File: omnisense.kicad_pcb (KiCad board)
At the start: 2 copper layers, 40 x 55 mm, 21 parts, among them J2 USB_C_Receptacle_USB2.0_16P, U1 ESP32-S3-WROOM-1, U3 TLV76133DCY

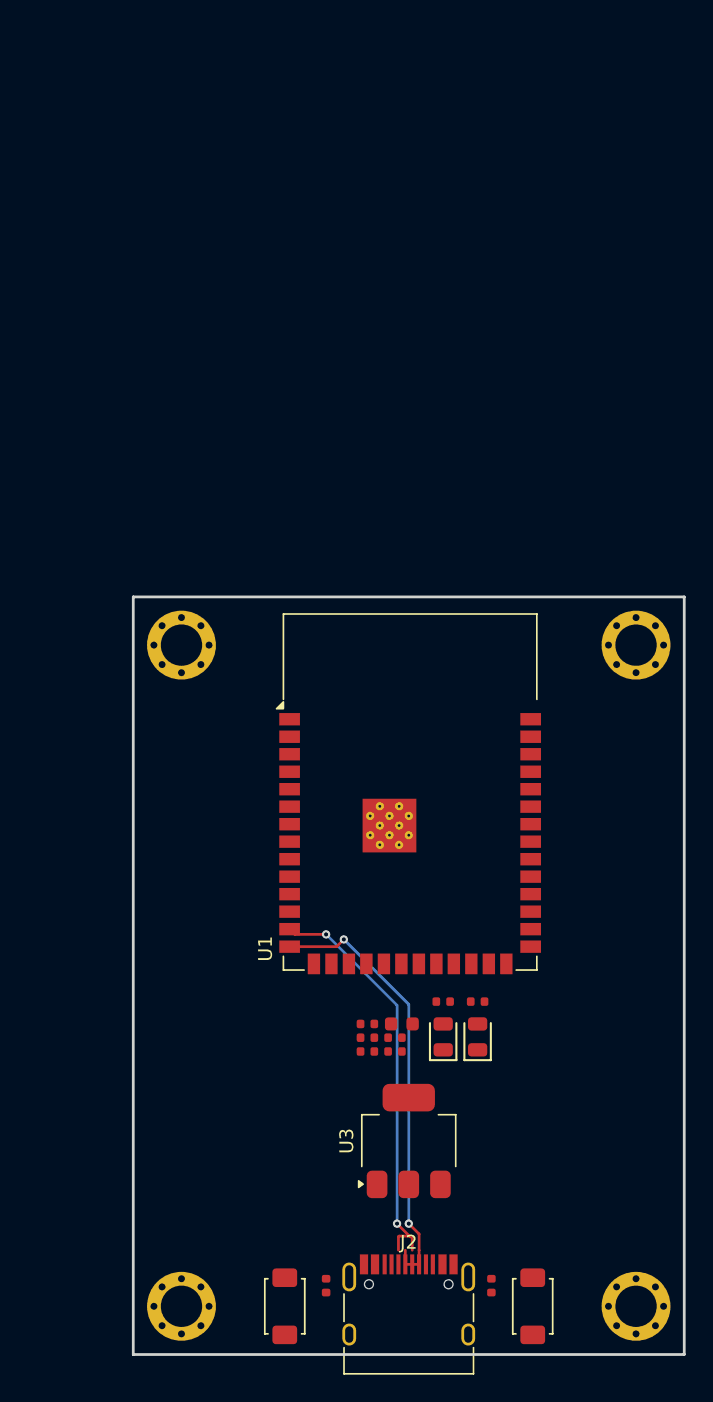
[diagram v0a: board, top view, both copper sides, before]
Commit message: lgtm
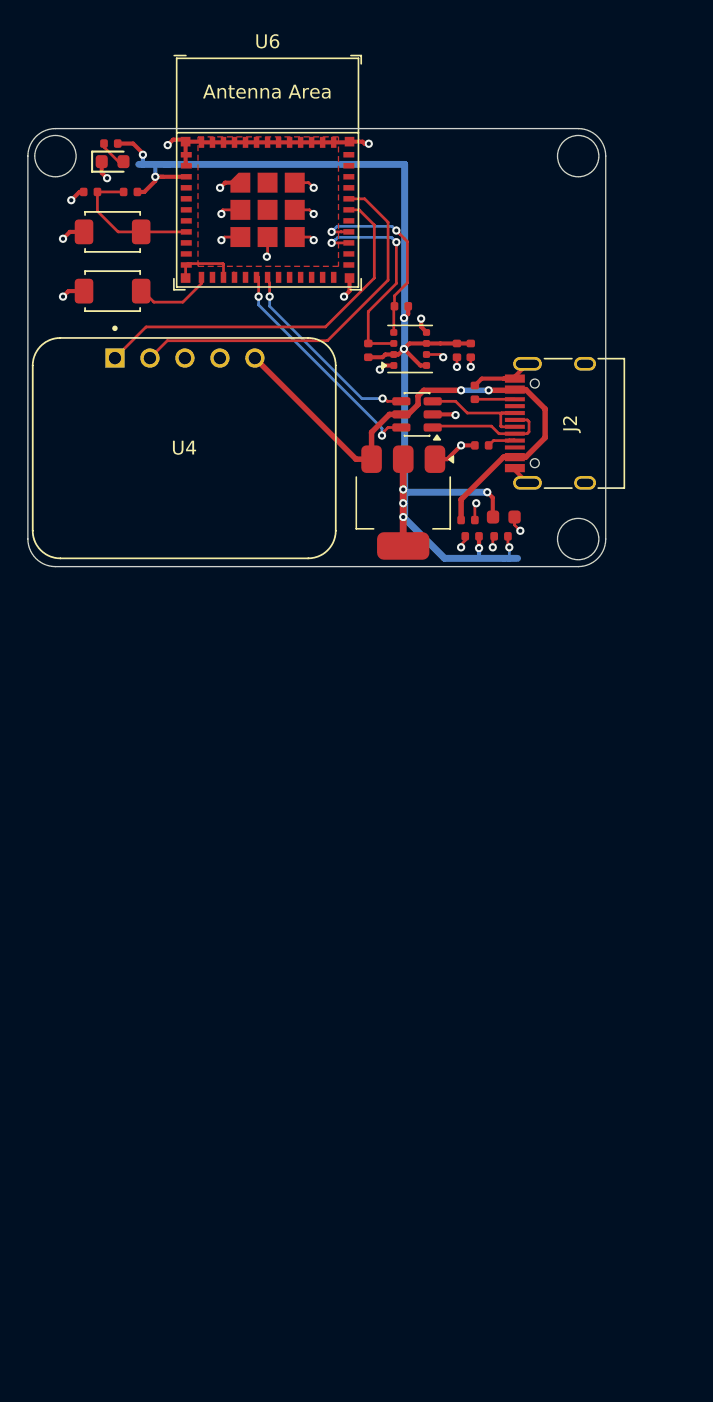
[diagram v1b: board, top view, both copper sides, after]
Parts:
- removed D2: White, PCM_JLCPCB:D_0805
- removed H1, H2, H3, H4: ~, PCM_JLCPCB:Hole, 3mm
- removed R4: 5.1kΩ, PCM_JLCPCB:R_0402
- added C6: 100nF, PCM_JLCPCB:C_0402, F.Cu at (163.5, 57.6)
- added C7: 100nF, PCM_JLCPCB:C_0402, F.Cu at (162.5, 57.6)
- added G***: LOGO, LOGO, F.Cu at (164.9, 50.3)
- added R6: 4.7kΩ, PCM_JLCPCB:R_0402, F.Cu at (158.5, 54.4)
- added R7: 4.7kΩ, PCM_JLCPCB:R_0402, F.Cu at (156.1, 57.6)
- added U2: BME680, Package_LGA:Bosch_LGA-8_3x3mm_P0.8mm_ClockwisePinNumbering, F.Cu at (159.1, 57.5)
- added U4: HLK-LD2410C, HLK-LD2410C:MODULE_HLK-LD2410C, F.Cu at (142.7, 64.7)
- added U6: ESP32-C6-MINI-1/U, PCM_Espressif:ESP32-C6-MINI-1, F.Cu at (148.8, 44.7)
- D1: footprint PCM_JLCPCB:D_0805 -> PCM_JLCPCB:D_0603
- R3: value 5.1kΩ -> 150Ω
- U1: value ESP32-S3-WROOM-1 -> USBLC6-2SC6; footprint RF_Module:ESP32-S3-WROOM-1 -> Package_TO_SOT_SMD:SOT-23-6
- moved S1 79.8 mm to (137.5, 53.3), turned to 0 degrees
- moved S2 79.0 mm to (137.5, 49.0), turned to 0 degrees
- moved D1 67.9 mm to (137.5, 43.9), turned to 0 degrees
- moved R3 66.8 mm to (137.4, 42.6)
- moved J2 66.2 mm to (170.8, 62.9), turned to 90 degrees
- moved C5 65.3 mm to (135.9, 46.1)
- moved R2 64.9 mm to (163.8, 60.6), turned to 90 degrees
- moved R5 62.8 mm to (138.8, 46.1), turned to 0 degrees
- moved R1 62.0 mm to (164.3, 64.5), turned to 180 degrees
- moved U3 46.4 mm to (158.6, 68.7), turned to -90 degrees
- moved C1 38.9 mm to (163.3, 69.9)
- moved C4 38.2 mm to (163.6, 71.1), turned to 180 degrees
- moved C2 37.7 mm to (165.7, 71.1), turned to 180 degrees
- moved C3 37.5 mm to (165.9, 69.7), turned to 0 degrees
- moved U1 27.4 mm to (159.6, 62.2), turned to 180 degrees
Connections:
- J2 pad A6: USB_D+ -> Net-(J2-D+-PadA6)
- J2 pad A7: USB_D- -> Net-(J2-D--PadA7)
- J2 pad B6: USB_D+ -> Net-(J2-D+-PadA6)
- J2 pad B7: USB_D- -> Net-(J2-D--PadA7)
- R3 pad 1: Net-(D1-Pad2) -> +3V3
- R3 pad 2: +3V3 -> Net-(D1-Pad2)
- U1 pad 1: GND -> Net-(J2-D--PadA7)
- U1 pad 2: +3V3 -> GND
- U1 pad 3: EN -> Net-(J2-D+-PadA6)
- U1 pad 4: unconnected-(U1-IO4-Pad4) -> USB_D+
- U1 pad 5: unconnected-(U1-IO5-Pad5) -> +5V
- U1 pad 6: unconnected-(U1-IO6-Pad6) -> USB_D-
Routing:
- net +3V3: track 0.00 -> 91.3 mm, vias 0 -> 10
- net GND: track 0.00 -> 61.3 mm, vias 0 -> 25
- net +5V: track 0.00 -> 40.0 mm, vias 0 -> 2
- net ESP_TX: track 0.00 -> 27.4 mm
- net ESP_RX: track 0.00 -> 27.2 mm
- net USB_D+: track 32.0 -> 14.7 mm
- net SDA: track 0.00 -> 16.3 mm, vias 0 -> 2
- net SCL: track 0.00 -> 14.4 mm, vias 0 -> 2
- net USB_D-: track 30.4 -> 17.1 mm
- net EN: track 0.00 -> 10.2 mm
- net Net-(J2-D+-PadA6): track 0.00 -> 9.31 mm
- net Net-(J2-D--PadA7): track 0.00 -> 9.14 mm
- net GPIO0: track 0.00 -> 5.87 mm
- net Net-(J2-CC2): track 0.00 -> 2.91 mm
- net Net-(J2-CC1): track 0.00 -> 2.62 mm
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- added copper zone on F.Cu, net GND
- added copper zone on In1.Cu, net GND
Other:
- board size 40 x 55 mm -> 42 x 31.8 mm
- copper layers 2 -> 4
- board text removed: "KEEP-OUT ZONE"
